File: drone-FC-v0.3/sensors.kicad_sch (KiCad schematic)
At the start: 14 parts, among them J2 Conn_01x04_Pin, U3 BMI088, U6 LIS3MDL, U7 MS5607-02BA

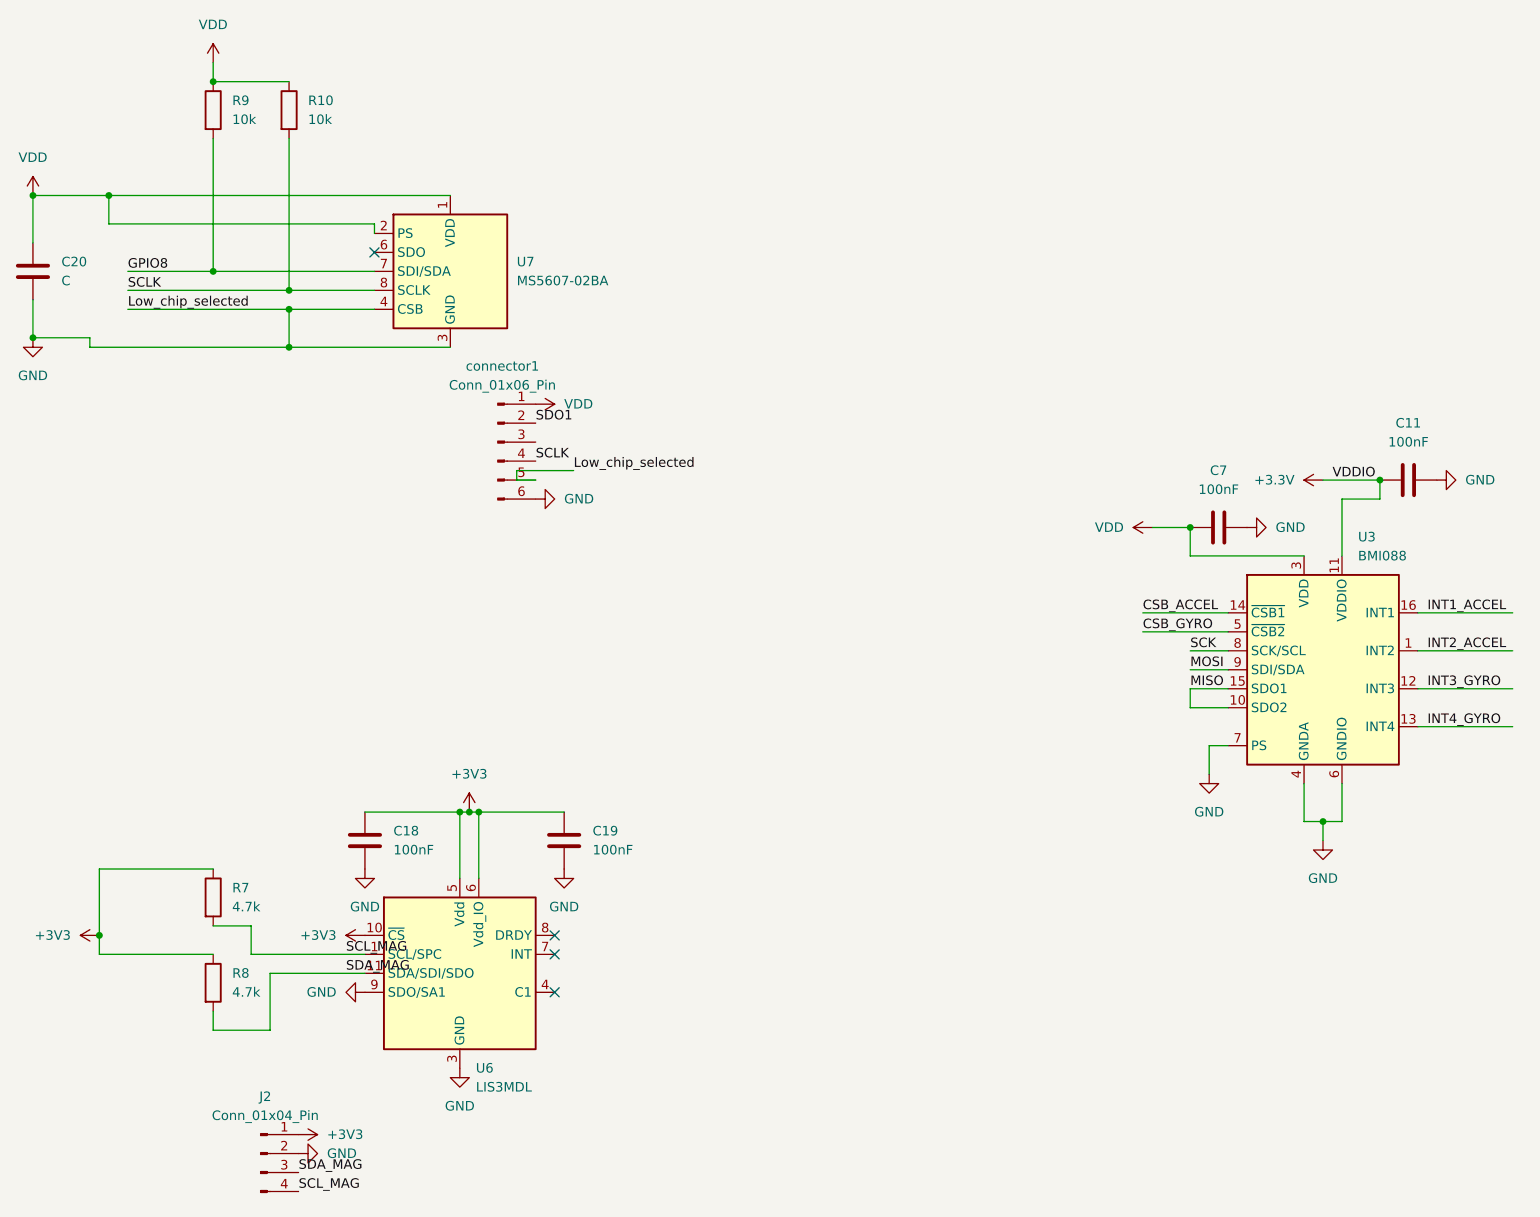
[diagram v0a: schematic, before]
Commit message: "global labels added"
"global labels added"
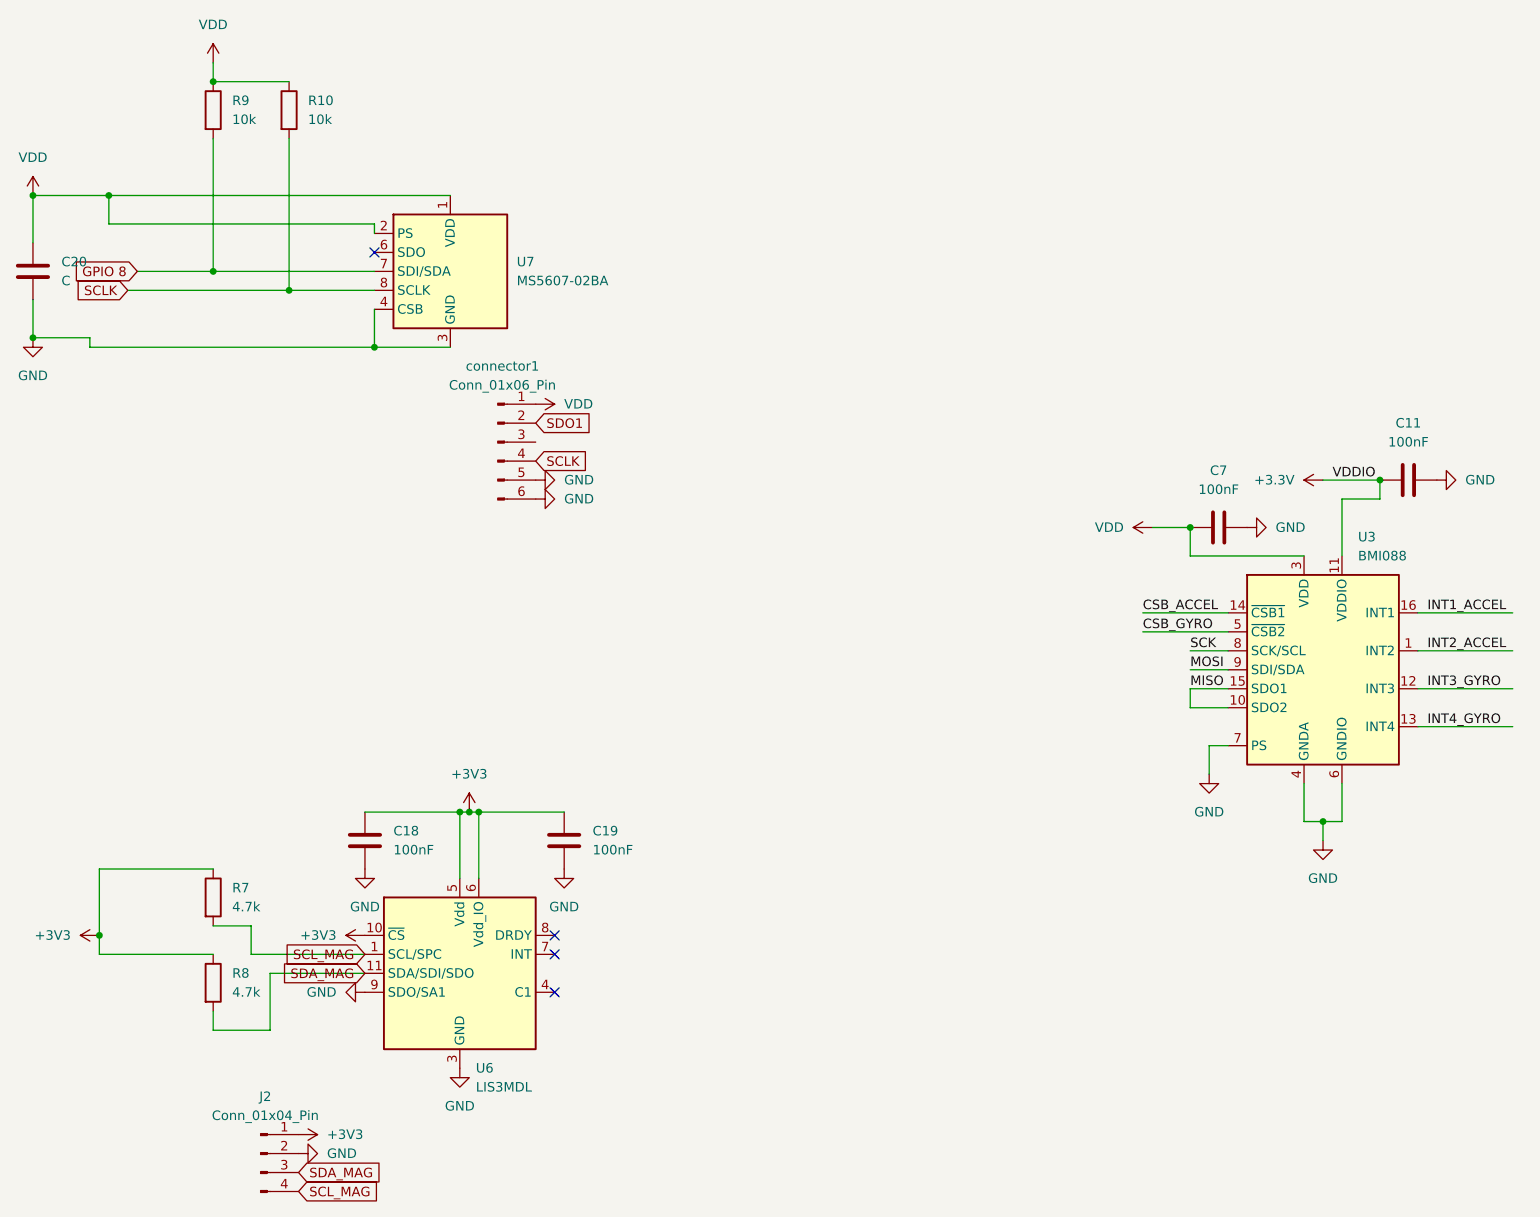
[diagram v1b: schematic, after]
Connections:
- net GPIO8 renamed GPIO 8
